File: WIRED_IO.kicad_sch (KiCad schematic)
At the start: 39 parts, among them J7 USB4085-GF-A_REVA4, J8 USB_A, J9 SM04B-GHS-TB(LF)(SN), J9C1 J9 female crimp contact, J9C2 J9 female crimp contact, J9C3 J9 female crimp contact, J9M1 J9 mating housing, 4-position, Q1 MMBT3904, Q2 MMBT3904, U32 TPD2E2U06DCK, U33 CP2102N-Axx-xQFN24, U34 TPD2E2U06DCK, U36 SN65HVD230

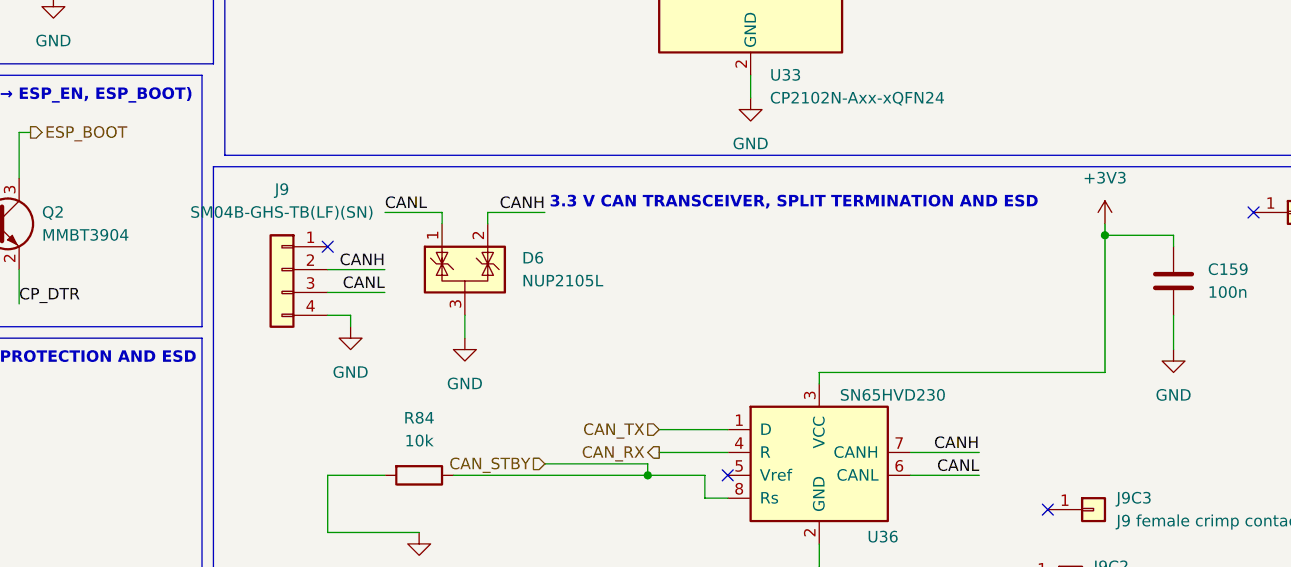
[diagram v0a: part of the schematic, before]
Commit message: the schematic is finished
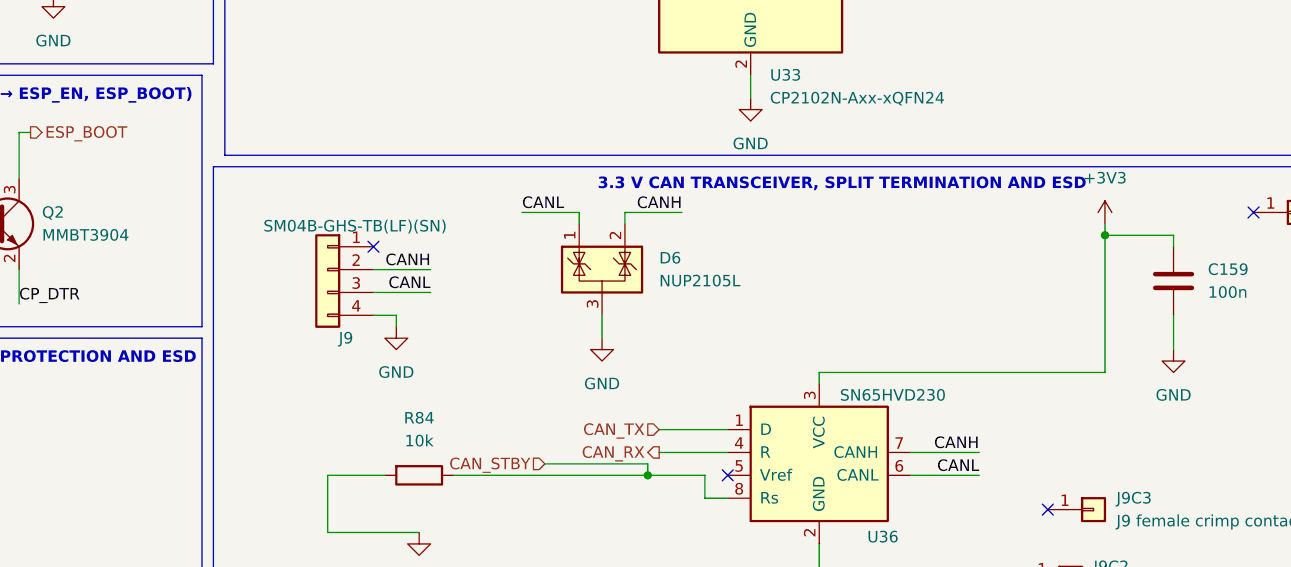
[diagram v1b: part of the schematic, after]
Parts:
- C153, C155: Notes (none) -> N/A
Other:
- moved on the sheet: D6, J9
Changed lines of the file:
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@@
 	(text "3.3 V CAN TRANSCEIVER, SPLIT TERMINATION AND ESD"
 		(exclude_from_sim no)
-		(at 188.976 115.824 0)
+		(at 194.31 113.792 0)
 		(effects
 			(font
@@
 	)
 	(no_connect
-		(at 137.16 120.65)
+		(at 142.24 120.65)
 	)
 	(no_connect
@@
 	(wire
 		(pts
-			(xy 152.4 128.27) (xy 152.4 130.81)
+			(xy 167.64 128.27) (xy 167.64 130.81)
 		)
 		(stroke
@@
 	(wire
 		(pts
-			(xy 137.16 123.19) (xy 143.51 123.19)
+			(xy 142.24 123.19) (xy 148.59 123.19)
 		)
 		(stroke
@@
 	(wire
 		(pts
-			(xy 139.7 128.27) (xy 139.7 129.54)
+			(xy 144.78 128.27) (xy 144.78 129.54)
 		)
 		(stroke
@@
 	(wire
 		(pts
-			(xy 154.94 116.84) (xy 161.29 116.84)
+			(xy 170.18 116.84) (xy 176.53 116.84)
 		)
 		(stroke
@@
 	(wire
 		(pts
-			(xy 149.86 116.84) (xy 143.51 116.84)
+			(xy 165.1 116.84) (xy 158.75 116.84)
 		)
 		(stroke
@@
 	(wire
 		(pts
-			(xy 137.16 125.73) (xy 143.51 125.73)
+			(xy 142.24 125.73) (xy 148.59 125.73)
 		)
 		(stroke
@@
 	(wire
 		(pts
-			(xy 149.86 118.11) (xy 149.86 116.84)
+			(xy 165.1 118.11) (xy 165.1 116.84)
 		)
 		(stroke
@@
 	(wire
 		(pts
-			(xy 137.16 128.27) (xy 139.7 128.27)
+			(xy 142.24 128.27) (xy 144.78 128.27)
 		)
 		(stroke
@@
 	(wire
 		(pts
-			(xy 154.94 118.11) (xy 154.94 116.84)
+			(xy 170.18 118.11) (xy 170.18 116.84)
 		)
 		(stroke
@@
 	)
 	(label "CANL"
-		(at 143.51 116.84 0)
+		(at 158.75 116.84 0)
 		(effects
 			(font
@@
 	)
 	(label "CANH"
-		(at 143.51 123.19 180)
+		(at 148.59 123.19 180)
 		(effects
 			(font
@@
 	)
 	(label "CANL"
-		(at 143.51 125.73 180)
+		(at 148.59 125.73 180)
 		(effects
 			(font
@@
 	)
 	(label "CANH"
-		(at 161.29 116.84 180)
+		(at 176.53 116.84 180)
 		(effects
 			(font
@@
 			)
 		)
-		(property "Notes" ""
+		(property "Notes" "N/A"
 			(at 222.25 26.67 0)
 			(hide yes)
@@
 	(symbol
 		(lib_id "Connector_Generic:Conn_01x04")
-		(at 132.08 123.19 0)
+		(at 137.16 123.19 0)
 		(mirror y)
 		(unit 1)
@@
 		(in_pos_files yes)
 		(dnp no)
-		(fields_autoplaced yes)
 		(property "Reference" "J9"
-			(at 132.08 114.3 0)
+			(at 139.192 130.81 0)
 			(show_name no)
 			(do_not_autoplace no)
@@
 		)
 		(property "Value" "SM04B-GHS-TB(LF)(SN)"
-			(at 132.08 116.84 0)
+			(at 140.208 118.364 0)
 			(show_name no)
 			(do_not_autoplace no)
@@
 		)
 		(property "Footprint" "Connector_JST:JST_GH_SM04B-GHS-TB_1x04-1MP_P1.25mm_Horizontal"
-			(at 132.08 123.19 0)
+			(at 137.16 123.19 0)
 			(hide yes)
 			(show_name no)
@@
 		)
 		(property "Datasheet" "https://www.jst-mfg.com/product/pdf/eng/eGH.pdf"
-			(at 132.08 123.19 0)
+			(at 137.16 123.19 0)
 			(hide yes)
 			(show_name no)
@@
 		)
 		(property "Description" "Generic connector, single row, 01x04, script generated (kicad-library-utils/schlib/autogen/connector/)"
-			(at 132.08 123.19 0)
+			(at 137.16 123.19 0)
 			(hide yes)
 			(show_name no)
@@
 		)
 		(property "DISTRIBUTOR_LINK" "https://www.mouser.com/ProductDetail/JST-Commercial/SM04B-GHS-TBLFSN?qs=QpmGXVUTftGayLYZQBIuZw%3D%3D"
-			(at 132.08 123.19 0)
+			(at 137.16 123.19 0)
 			(hide yes)
 			(show_name no)
@@
 		)
 		(property "MPN" "SM04B-GHS-TB(LF)(SN)"
-			(at 132.08 123.19 0)
+			(at 137.16 123.19 0)
 			(hide yes)
 			(show_name no)
@@
 		)
 		(property "KLC_S3.3" ""
-			(at 132.08 123.19 0)
+			(at 137.16 123.19 0)
 			(hide yes)
 			(show_name no)
@@
 		)
 		(property "KLC_S4.1" ""
-			(at 132.08 123.19 0)
+			(at 137.16 123.19 0)
 			(hide yes)
 			(show_name no)
@@
 		)
 		(property "KLC_S4.2_DVDD" ""
-			(at 132.08 123.19 0)
+			(at 137.16 123.19 0)
 			(hide yes)
 			(show_name no)
@@
 		)
 		(property "KLC_S4.2_VREG_LX" ""
-			(at 132.08 123.19 0)
+			(at 137.16 123.19 0)
 			(hide yes)
 			(show_name no)
@@
 		)
 		(property "Notes" "Frozen Rev-A pinout: pin 1 NC, pin 2 CANH, pin 3 CANL, pin 4 GND. Mates GHR-04V-S. Fit three SSHL-002T-P0.2 contacts in cavities 2–4; cavity 1 remains empty."
-			(at 132.08 123.19 0)
+			(at 137.16 123.19 0)
 			(hide yes)
 			(show_name no)
@@
 		)
 		(property "MANUFACTURER" "JST"
-			(at 132.08 123.19 0)
+			(at 137.16 123.19 0)
 			(hide yes)
 			(show_name no)
@@
 		)
 		(property "TUNING_ALTERNATIVES" ""
-			(at 132.08 123.19 0)
+			(at 137.16 123.19 0)
 			(hide yes)
 			(show_name no)
@@
 	(symbol
 		(lib_id "Power_Protection:NUP2105L")
-		(at 152.4 123.19 0)
+		(at 167.64 123.19 0)
 		(unit 1)
 		(body_style 1)
@@
 		(fields_autoplaced yes)
 		(property "Reference" "D6"
-			(at 158.75 121.9199 0)
+			(at 173.99 121.9199 0)
 			(show_name no)
 			(do_not_autoplace no)
@@
 		)
 		(property "Value" "NUP2105L"
-			(at 158.75 124.4599 0)
+			(at 173.99 124.4599 0)
 			(show_name no)
 			(do_not_autoplace no)
@@
 		)
 		(property "Footprint" "Package_TO_SOT_SMD:SOT-23"
-			(at 158.115 124.46 0)
+			(at 173.355 124.46 0)
 			(hide yes)
 			(show_name no)
@@
 		)
 		(property "Datasheet" "https://www.onsemi.com/pdf/datasheet/nup2105l-d.pdf"
-			(at 155.575 120.015 0)
+			(at 170.815 120.015 0)
 			(hide yes)
 			(show_name no)
@@
 		)
 		(property "Description" "Dual Line CAN Bus Protector, 24Vrwm"
-			(at 152.4 123.19 0)
+			(at 167.64 123.19 0)
 			(hide yes)
 			(show_name no)
@@
 		)
 		(property "DISTRIBUTOR_LINK" "https://www.mouser.com/ProductDetail/onsemi/NUP2105LT1G?qs=ZXBb0xZ9WeDHmiHN%252BYKtYA%3D%3D"
-			(at 152.4 123.19 0)
+			(at 167.64 123.19 0)
 			(hide yes)
 			(show_name no)
@@
 		)
 		(property "MPN" "NUP2105LT1G"
-			(at 152.4 123.19 0)
+			(at 167.64 123.19 0)
 			(hide yes)
 			(show_name no)
@@
 		)
 		(property "KLC_S3.3" ""
-			(at 152.4 123.19 0)
+			(at 167.64 123.19 0)
 			(hide yes)
 			(show_name no)
@@
 		)
 		(property "KLC_S4.1" ""
-			(at 152.4 123.19 0)
+			(at 167.64 123.19 0)
 			(hide yes)
 			(show_name no)
@@
 		)
 		(property "KLC_S4.2_DVDD" ""
-			(at 152.4 123.19 0)
+			(at 167.64 123.19 0)
 			(hide yes)
 			(show_name no)
@@
 		)
 		(property "KLC_S4.2_VREG_LX" ""
-			(at 152.4 123.19 0)
+			(at 167.64 123.19 0)
 			(hide yes)
 			(show_name no)
@@
 		)
 		(property "Notes" "N/A"
-			(at 152.4 123.19 0)
+			(at 167.64 123.19 0)
 			(hide yes)
 			(show_name no)
@@
 		)
 		(property "MANUFACTURER" "onsemi"
-			(at 152.4 123.19 0)
+			(at 167.64 123.19 0)
 			(hide yes)
 			(show_name no)
@@
 		)
 		(property "TUNING_ALTERNATIVES" ""
-			(at 152.4 123.19 0)
+			(at 167.64 123.19 0)
 			(hide yes)
 			(show_name no)
@@
 	(symbol
 		(lib_id "power:GND")
-		(at 152.4 130.81 0)
+		(at 167.64 130.81 0)
 		(unit 1)
 		(body_style 1)
@@
 		(fields_autoplaced yes)
 		(property "Reference" "#PWR0205"
-			(at 152.4 137.16 0)
+			(at 167.64 137.16 0)
 			(hide yes)
 			(show_name no)
@@
 		)
 		(property "Value" "GND"
-			(at 152.4 135.89 0)
+			(at 167.64 135.89 0)
 			(show_name no)
 			(do_not_autoplace no)
@@
 		)
 		(property "Footprint" ""
-			(at 152.4 130.81 0)
+			(at 167.64 130.81 0)
 			(hide yes)
 			(show_name no)
@@
 		)
 		(property "Datasheet" ""
-			(at 152.4 130.81 0)
+			(at 167.64 130.81 0)
 			(hide yes)
 			(show_name no)
@@
 		)
 		(property "Description" "Power symbol creates a global label with name \"GND\" , ground"
-			(at 152.4 130.81 0)
+			(at 167.64 130.81 0)
 			(hide yes)
 			(show_name no)
@@
 			)
 		)
-		(property "Notes" ""
+		(property "Notes" "N/A"
 			(at 194.31 26.67 0)
 			(hide yes)
@@
 	(symbol
 		(lib_id "power:GND")
-		(at 139.7 129.54 0)
+		(at 144.78 129.54 0)
 		(unit 1)
 		(body_style 1)
@@
 		(fields_autoplaced yes)
 		(property "Reference" "#PWR0206"
-			(at 139.7 135.89 0)
+			(at 144.78 135.89 0)
 			(hide yes)
 			(show_name no)
@@
 		)
 		(property "Value" "GND"
-			(at 139.7 134.62 0)
+			(at 144.78 134.62 0)
 			(show_name no)
 			(do_not_autoplace no)
@@
 		)
 		(property "Footprint" ""
-			(at 139.7 129.54 0)
+			(at 144.78 129.54 0)
 			(hide yes)
 			(show_name no)
@@
 		)
 		(property "Datasheet" ""
-			(at 139.7 129.54 0)
+			(at 144.78 129.54 0)
 			(hide yes)
 			(show_name no)
@@
 		)
 		(property "Description" "Power symbol creates a global label with name \"GND\" , ground"
-			(at 139.7 129.54 0)
+			(at 144.78 129.54 0)
 			(hide yes)
 			(show_name no)
